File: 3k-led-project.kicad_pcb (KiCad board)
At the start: 2 copper layers, 25 parts, among them SW1 SW_Push, U1 PRTR5V0U2X, U2 ATmega32U2-A, Y1 Crystal_GND24_Small

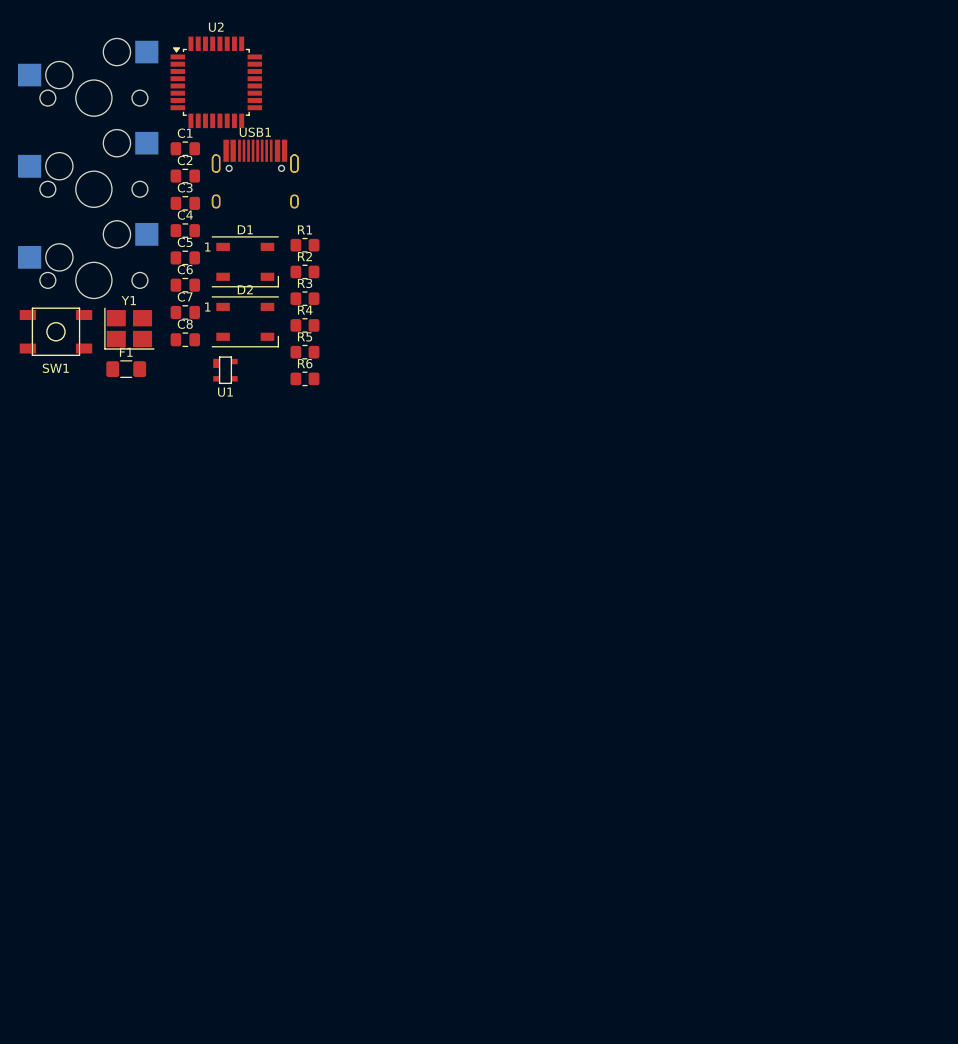
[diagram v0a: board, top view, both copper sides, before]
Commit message: pcb
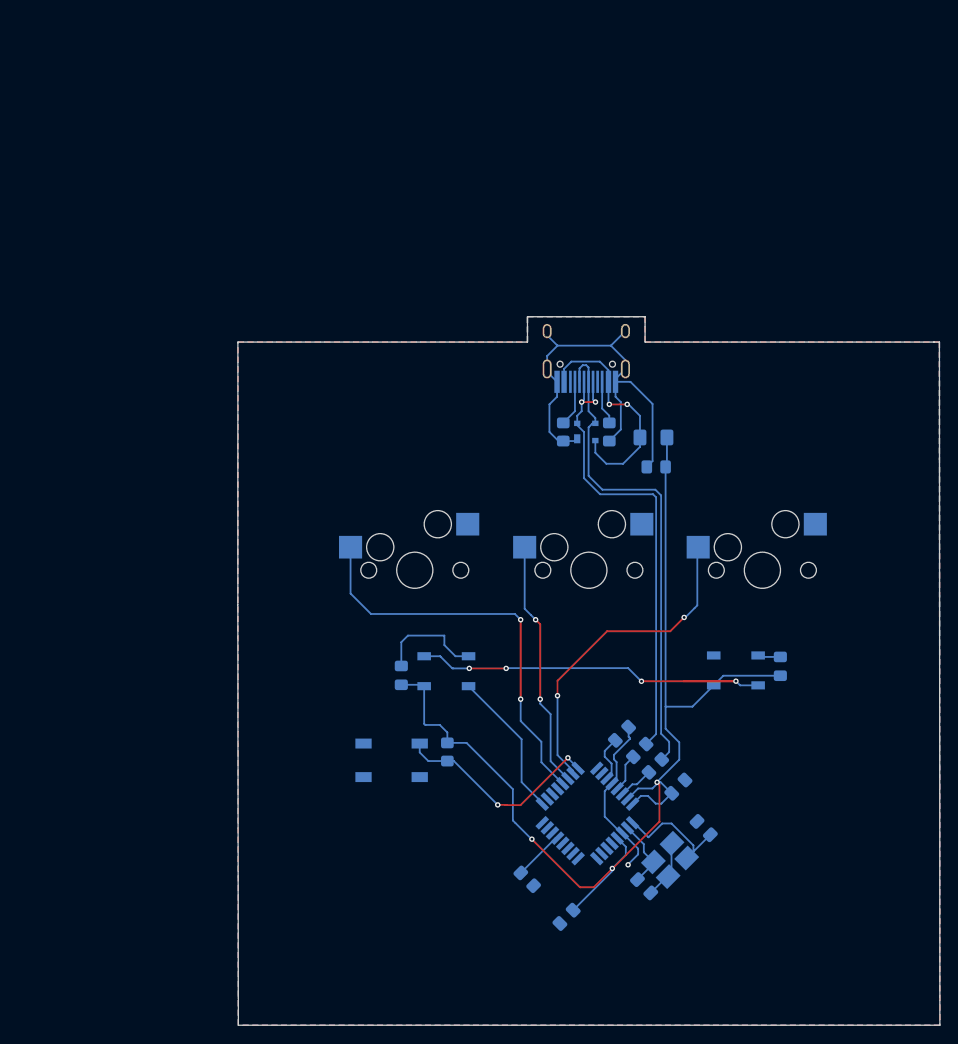
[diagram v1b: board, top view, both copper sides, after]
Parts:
- C1, C2, C3, C4, C5, C6, C7, C8, D1, D2, F1, R1, R2, R3, R4, R5, R6, SW1, U1, U2, USB1, Y1: moved to B.Cu
- moved C1 94.6 mm to (117.7, 146.2), turned to -135 degrees
- moved U2 90.5 mm to (120.0, 134.8), turned to 135 degrees
- moved MX1 90.3 mm to (139.3, 108.0)
- moved C2 86.6 mm to (130.0, 131.8), turned to 45 degrees
- moved C5 85.0 mm to (132.8, 136.4), turned to -45 degrees
- moved Y1 83.6 mm to (129.1, 139.9), turned to 45 degrees
- moved C6 83.4 mm to (126.3, 142.8), turned to 135 degrees
- moved C3 75.8 mm to (123.8, 126.0), turned to -135 degrees
- moved C8 74.9 mm to (141.3, 118.5), turned to -90 degrees
- moved R1 69.2 mm to (127.5, 129.5), turned to -135 degrees
- moved MX2 68.9 mm to (120.2, 108.0)
- moved D2 66.4 mm to (136.4, 119.0)
- moved R2 64.4 mm to (125.8, 127.8), turned to -135 degrees
- moved R6 60.4 mm to (113.4, 142.1), turned to -45 degrees
- moved SW1 60.1 mm to (98.4, 128.9), turned to 180 degrees
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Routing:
- net +5V: track 0.00 -> 126.8 mm, vias 0 -> 3
- net GND: track 0.00 -> 89.4 mm, vias 0 -> 1
- net D-: track 0.00 -> 54.2 mm
- net D+: track 0.00 -> 51.6 mm, vias 0 -> 2
- net COL2: track 0.00 -> 45.1 mm, vias 0 -> 2
- net Net-(D1-DOUT): track 0.00 -> 44.0 mm, vias 0 -> 4
- net COL0: track 0.00 -> 36.2 mm, vias 0 -> 2
- net COL1: track 0.00 -> 27.5 mm, vias 0 -> 2
- net VCC: track 0.00 -> 25.9 mm, vias 0 -> 2
- net Net-(U2-PC1/~{RESET}): track 0.00 -> 23.6 mm, vias 0 -> 2
- net UNDERGLOWLED: track 0.00 -> 16.4 mm
- net XTAL1: track 0.00 -> 14.4 mm
- net XTAL2: track 0.00 -> 7.62 mm
- net Net-(U2-~{HWB}/PD7): track 0.00 -> 5.65 mm
- net Net-(USB1-CC1): track 0.00 -> 5.58 mm
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- added copper zone on B.Cu, net GND
- added copper zone on F.Cu, net GND
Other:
- board outline added: 77.5 x 78.2 mm
